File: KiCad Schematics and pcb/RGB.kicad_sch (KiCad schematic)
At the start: 15 parts, among them J5 Screw_Terminal_01x06, J6 Screw_Terminal_01x03, Q3 DMN4035L-7, Q4 DMN4035L-7, Q5 DMN4035L-7, Q6 DMN4035L-7, Q7 DMN4035L-7, Q8 2N7002NXAKR

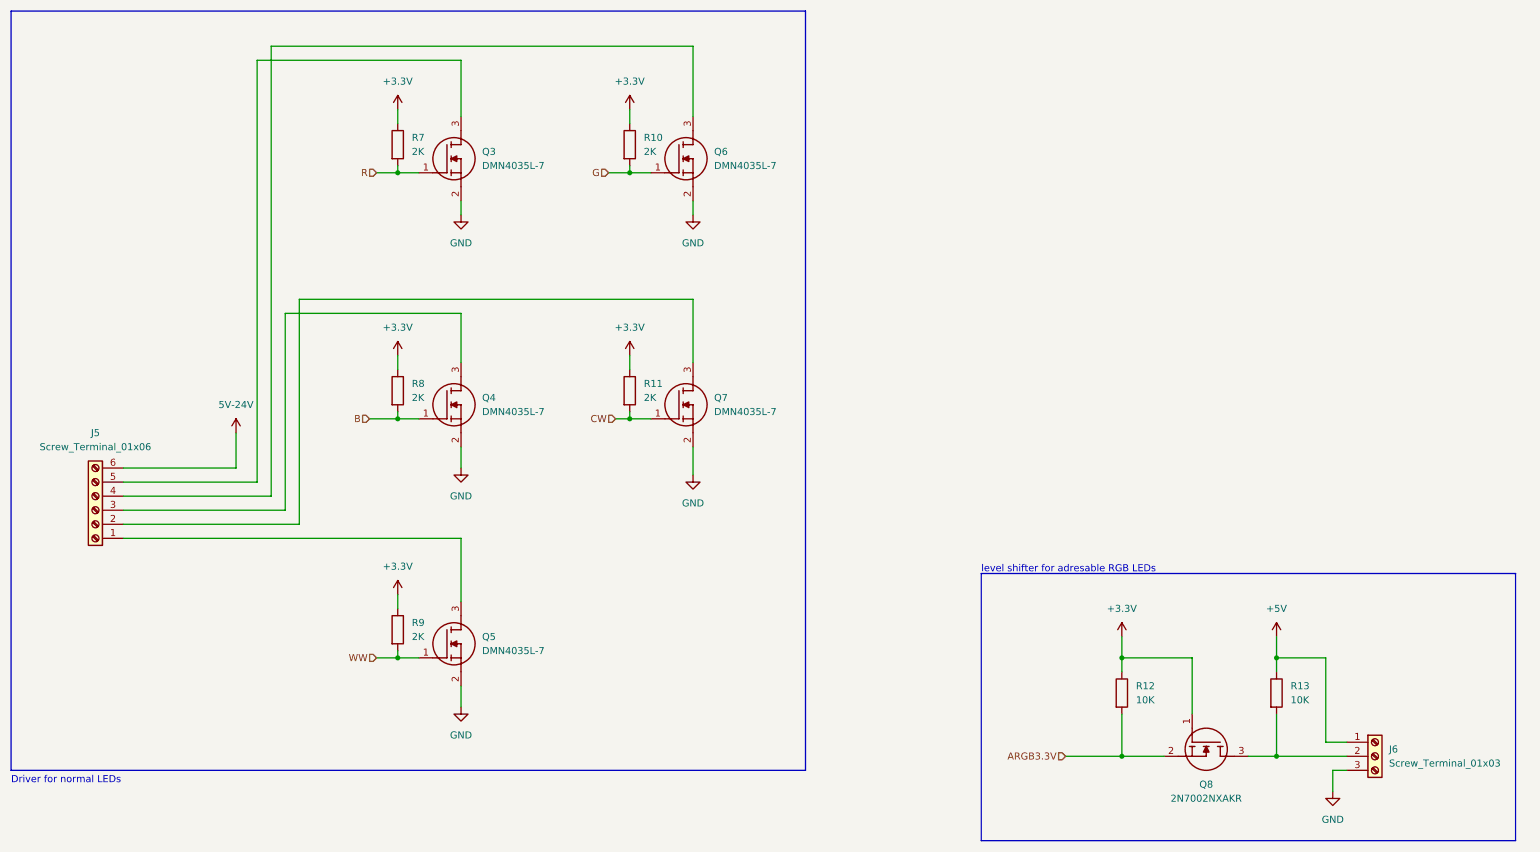
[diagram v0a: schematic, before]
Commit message: v0.1
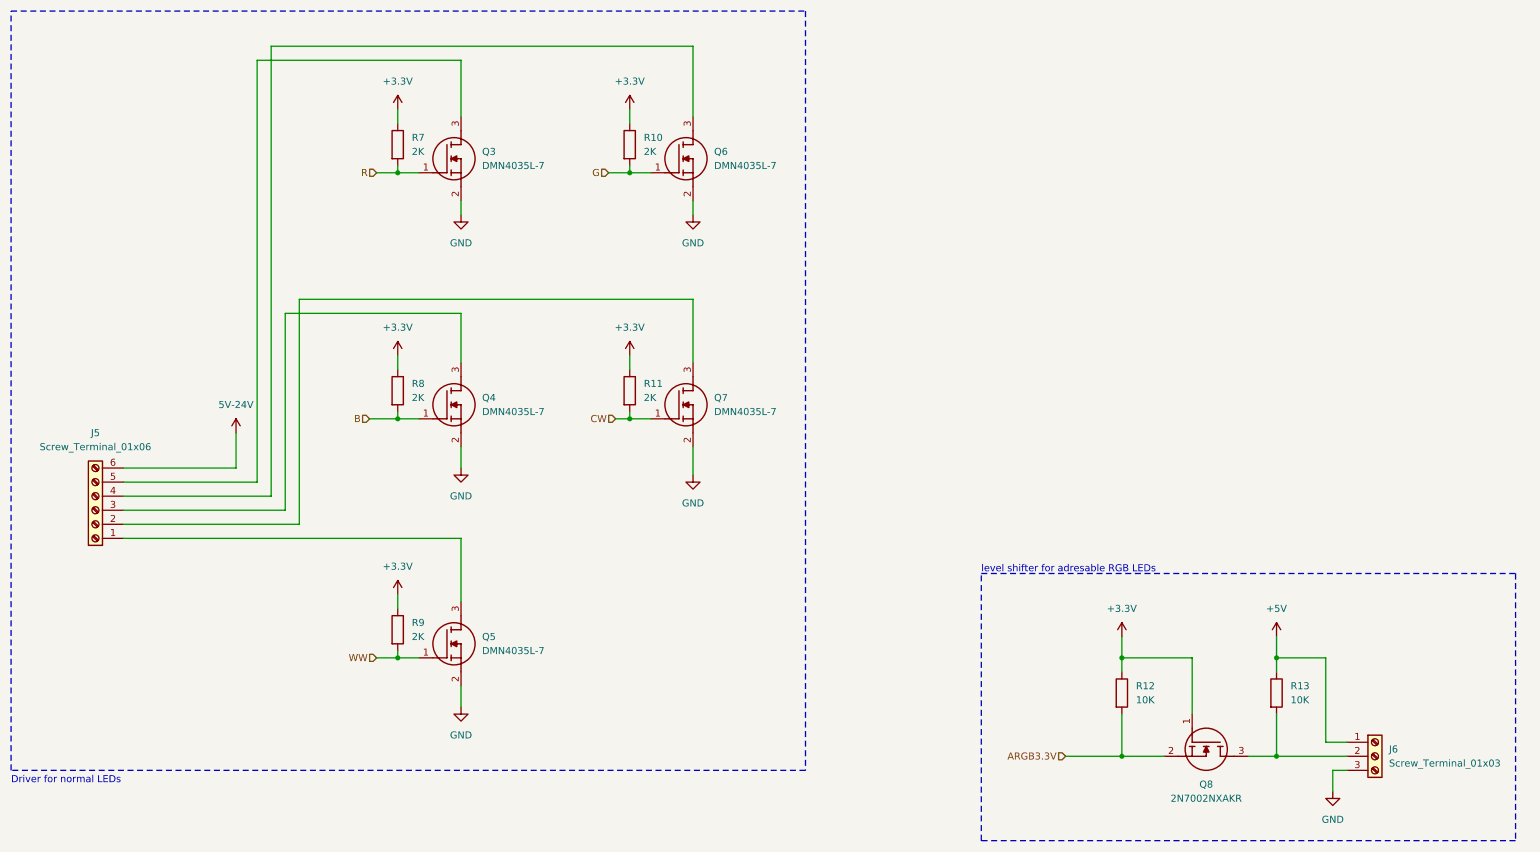
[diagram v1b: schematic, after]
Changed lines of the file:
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@@
   )
   (rectangle (start 187.96 114.3) (end 284.48 162.56)
-    (stroke (width 0) (type default))
+    (stroke (width 0) (type dash))
     (fill (type none))
   )
   (rectangle (start 12.7 12.7) (end 156.21 149.86)
-    (stroke (width 0) (type default))
+    (stroke (width 0) (type dash))
     (fill (type none))
   )
